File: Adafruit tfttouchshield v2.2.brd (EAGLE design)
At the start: 70.4 x 54.4 mm, 41 parts, among them IC4 MIC5225-3.3, IC5 AXP803, Q2 BSS138, Q3 BSS138, Q4 BSS138, SW1 SPST_TACT-EVQQ2, U3 74HC4050

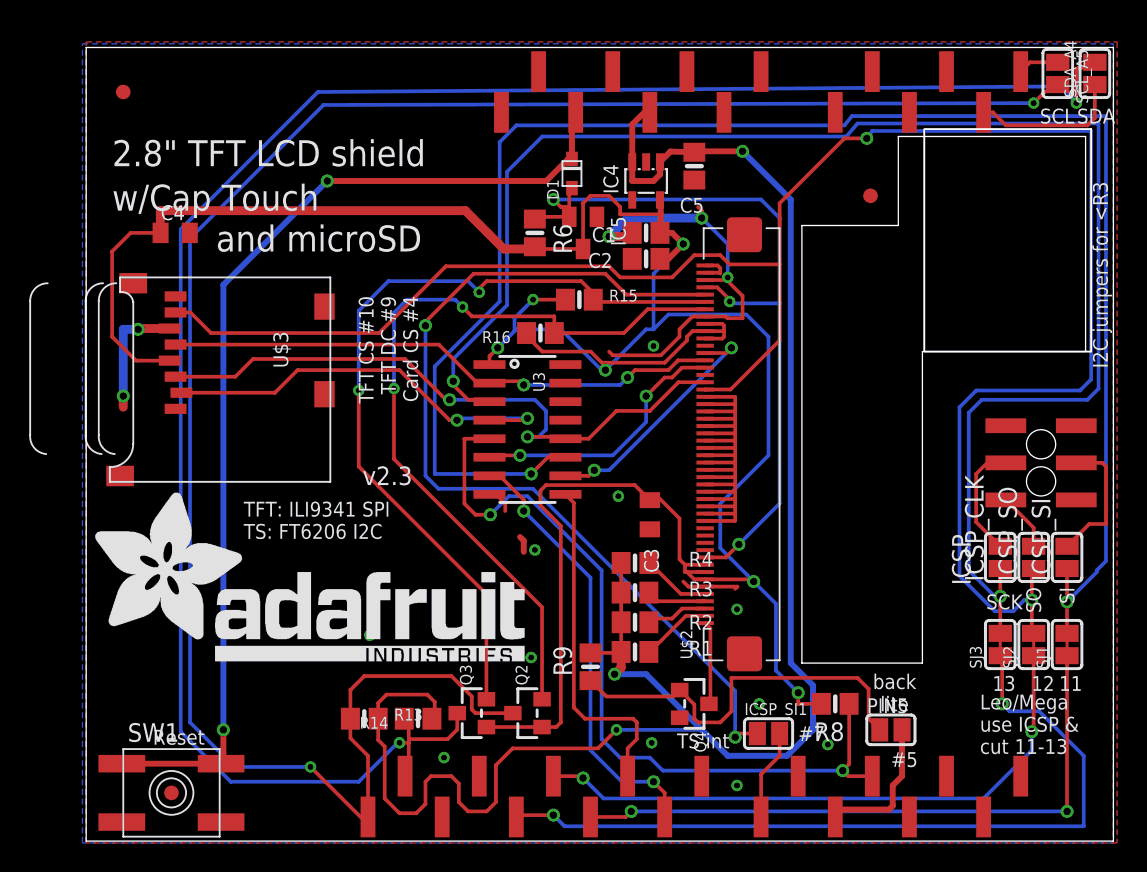
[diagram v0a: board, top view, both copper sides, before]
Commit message: Updated to latest versions
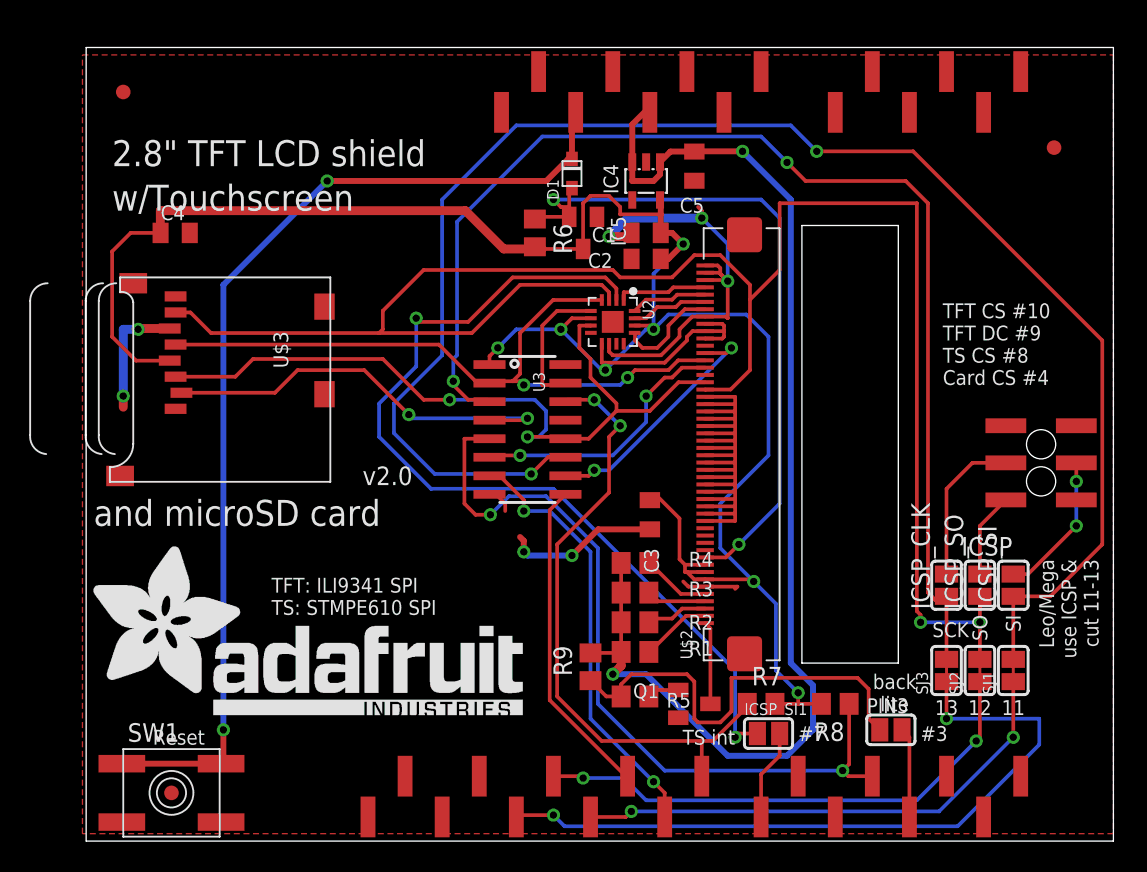
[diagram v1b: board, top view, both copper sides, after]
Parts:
- removed Q2, Q3, Q4: BSS138, microbuilder:SOT23-WIDE
- removed R13, R14, R15, R16: 10K, microbuilder:0805-NO
- removed SCL_A5, SDA_A4: (no value), microbuilder:SOLDERJUMPER_REFLOW_NOPASTE
- added Q1: MMBT2222, transistor-neu-to92:SOT23-BEC
- added R5: 1K, rcl:R0805
- added R7: 10K, rcl:R0805
- added U2: STMPE610, microbuilder:QFN16_3MM
- C1, C2, C5: device microbuilder:0805-NO -> adafruit:C0805K
- R1, R2, R3, R4, R6, R8: device microbuilder:0805-NO -> rcl:R0805
- R9: value 2.2K -> 1K; device microbuilder:0805-NO -> rcl:R0805
- U$2: value 2.8" TFT + CTP -> DISP_LCD_1.28IN_240X320_50PIN
- moved U$10 13.0 mm to (66.3, 47.5)
- moved ICSP_SI 4.15 mm to (63.5, 17.5)
- moved ICSP_SO 4.15 mm to (61.2, 17.5)
- moved ICSP_CLK 4.15 mm to (58.9, 17.5)
- moved SJ1 4.09 mm to (63.5, 11.7)
- moved SJ2 4.09 mm to (61.2, 11.7)
- moved SJ3 4.09 mm to (58.9, 11.7)
- moved U$20 3.69 mm to (0.25, 8.64)
- renumbered PIN5 to PIN3
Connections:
- removed net N$17: SDA_A4.1, U$17.A4
- removed net N$18: SCL_A5.1, U$17.A5
- removed net SCL_3V: Q2.2, R16.1, U$2.44
- removed net SCL_5V: Q2.3, R13.1, SCL_A5.2, U$17.SCL
- removed net SDA_3V: Q3.2, R15.2, U$2.45
- removed net SDA_5V: Q3.3, R14.2, SDA_A4.2, U$17.SDA
- removed net TP_IRQ: ICSP_SI1.1, U$2.46
- new net N$16: Q1.B, R5.2
- new net RT_CS_3V: U2.5, U3.15
- new net RT_CS_5V: R7.1, U$17.D8, U3.14
- new net TS_INT: ICSP_SI1.1, U2.2
- new net XL: U$2.46, U2.16
- new net XR: U$2.44, U2.13
- new net YD: U$2.45, U2.15
- new net YU: U$2.47, U2.1
- net +5V: no longer R13.2, R14.1
- net GND: now also Q1.E, U2.10; no longer Q4.2
- net MISO: now also U2.3
- net MOSI_3V: now also U2.7
- net N$1: now also Q1.C; no longer Q4.3
- net N$5: now also R5.1; no longer Q4.1
- net N$7: now also U$17.D3; no longer U$17.D5
- net SCLK_3V: now also U2.4
- net TFT_RST: no longer U$2.47
- net VCC: now also R7.2, U2.14, U2.6, U2.9; no longer Q2.1, Q3.1, R15.1, R16.2
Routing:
- net SCL_5V: track 135.2 -> 0.00 mm, vias 2 -> 0
- net SDA_5V: track 131.3 -> 0.00 mm, vias 2 -> 0
- net TP_IRQ: track 63.8 -> 0.00 mm, vias 2 -> 0
- net TS_INT: track 0.00 -> 62.6 mm, vias 0 -> 2
- net SDA_3V: track 56.4 -> 0.00 mm, vias 2 -> 0
- net SCL_3V: track 54.7 -> 0.00 mm, vias 2 -> 0
- net RT_CS_5V: track 0.00 -> 42.7 mm, vias 0 -> 2
- net +5V: track 125.1 -> 83.2 mm, vias 3 -> 2
- net VCC: track 191.3 -> 157.1 mm, vias 6 -> 7
- net SCLK_5V: track 106.9 -> 83.3 mm
- net N$17: track 10.5 -> 0.00 mm
- net GND: track 47.5 -> 57.9 mm, vias 16 -> 7
- net SCLK_3V: track 38.2 -> 48.3 mm
- net RT_CS_3V: track 0.00 -> 9.70 mm
- net N$15: track 43.5 -> 35.0 mm
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- removed copper zone on layer 16, net GND
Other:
- outline, holes or cut-outs redrawn
- board text added: "#3"
- board text added: "TFT CS #10 TFT DC #9 TS CS #8 Card CS #4"
- board text added: "TFT: ILI9341 SPI TS: STMPE610 SPI"
- board text added: "and microSD card"
- board text added: "v2.0"
- board text added: "w/Touchscreen"
- board text removed: "#5"
- board text removed: "I2C jumpers for <R3"
- board text removed: "SCL"
- board text removed: "SDA"
- board text removed: "TFT CS #10 TFT DC #9 Card CS #4"
- board text removed: "TFT: ILI9341 SPI TS: FT6206 I2C"
- board text removed: "and microSD"
- board text removed: "v2.3"
- board text removed: "w/Cap Touch"
